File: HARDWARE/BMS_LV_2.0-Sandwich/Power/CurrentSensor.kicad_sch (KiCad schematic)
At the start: 11 parts, among them U5 ACHS-7123

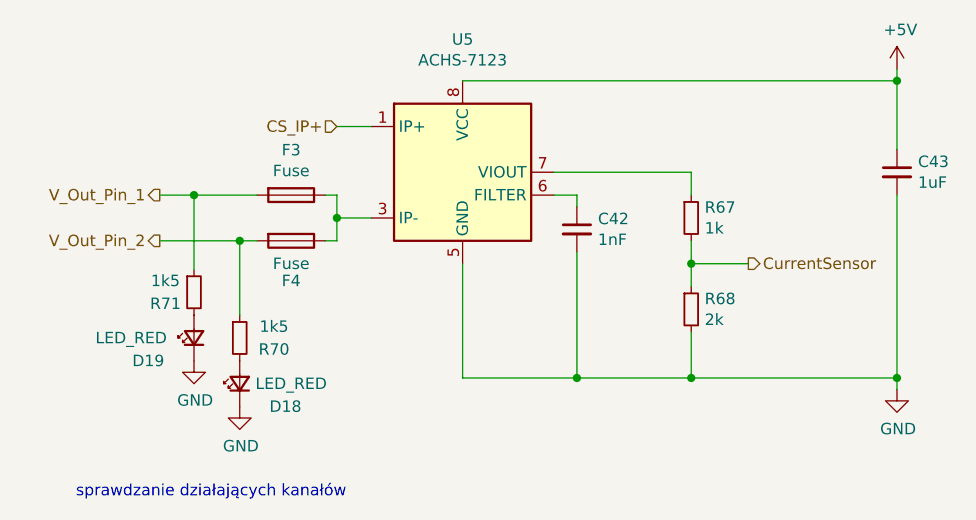
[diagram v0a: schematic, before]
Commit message: Wersja obu plytek gotowa do sprawdzenia
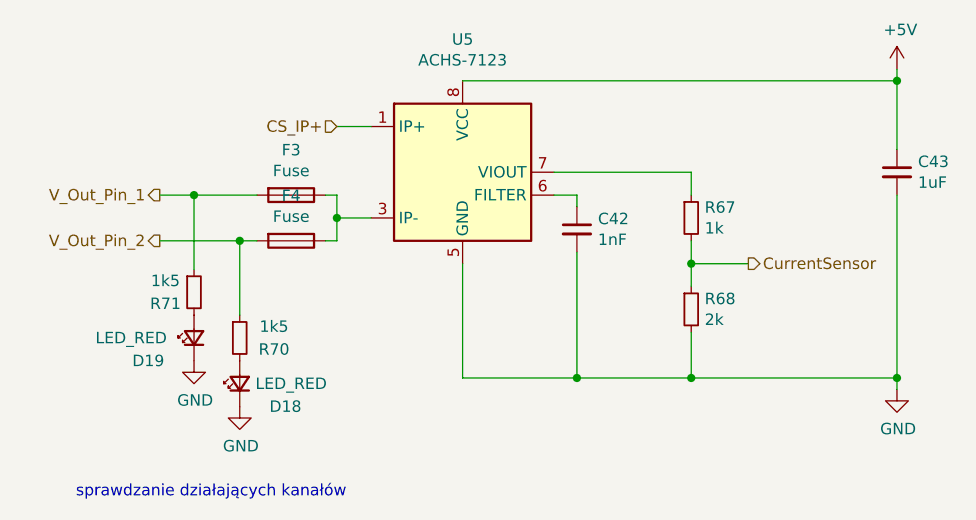
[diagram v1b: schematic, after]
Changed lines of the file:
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@@
+	)
+	(symbol
+		(lib_id "Device:Fuse")
+		(at 118.11 101.6 270)
+		(unit 1)
+		(exclude_from_sim no)
+		(in_bom yes)
+		(on_board yes)
+		(dnp no)
+		(property "Reference" "F4"
+			(at 118.11 96.5962 90)
+			(effects
+				(font
+					(size 1.27 1.27)
+				)
+			)
+		)
+		(property "Value" "Fuse"
+			(at 118.11 98.9076 90)
+			(effects
+				(font
+					(size 1.27 1.27)
+				)
+			)
+		)
+		(property "Footprint" "footprints:FUSC6125X279N"
+			(at 118.11 99.822 90)
+			(effects
+				(font
+					(size 1.27 1.27)
+				)
+				(hide yes)
+			)
+		)
+		(property "Datasheet" "https://www.mouser.pl/ProductDetail/Bel-Fuse/0680L9100-05?qs=XeJtXLiO41RjXNhvn3uPUw%3D%3D"
+			(at 118.11 101.6 0)
+			(effects
+				(font
+					(size 1.27 1.27)
+				)
+				(hide yes)
+			)
+		)
+		(property "Description" "500A interrupt fuse"
+			(at 118.11 101.6 0)
+			(effects
+				(font
+					(size 1.27 1.27)
+				)
+				(hide yes)
+			)
+		)
+		(property "Part Number" "0680L9100-05 "
+			(at 118.11 101.6 0)
+			(effects
+				(font
+					(size 1.27 1.27)
+				)
+				(hide yes)
+			)
+		)
+		(pin "2"
+		)
+		(pin "1"
+		)
+		(instances
+			(project "BMS_LV_2022"
+				(path "/fb6504b5-591d-4b10-ab86-0c46f59e8b7d/00000000-0000-0000-0000-000062c2dd72"
+					(reference "F4")
+					(unit 1)
+				)
+			)
+		)
 	)
 	(symbol
@@
 					(unit 1)
 				)
-			)
-		)
-	)
-	(symbol
-		(lib_id "Device:Fuse")
-		(at 118.11 101.6 270)
-		(unit 1)
-		(exclude_from_sim no)
-		(in_bom yes)
-		(on_board yes)
-		(dnp no)
-		(property "Reference" "F4"
-			(at 118.11 106.045 90)
-			(effects
-				(font
-					(size 1.27 1.27)
-				)
-			)
-		)
-		(property "Value" "Fuse"
-			(at 118.11 104.14 90)
-			(effects
-				(font
-					(size 1.27 1.27)
-				)
-			)
-		)
-		(property "Footprint" "footprints:FUSC6125X279N"
-			(at 118.11 99.822 90)
-			(effects
-				(font
-					(size 1.27 1.27)
-				)
-				(hide yes)
-			)
-		)
-		(property "Datasheet" "https://www.mouser.pl/ProductDetail/Bel-Fuse/0680L9100-05?qs=XeJtXLiO41RjXNhvn3uPUw%3D%3D"
-			(at 118.11 101.6 0)
-			(effects
-				(font
-					(size 1.27 1.27)
-				)
-				(hide yes)
-			)
-		)
-		(property "Description" "500A interrupt fuse"
-			(at 118.11 101.6 0)
-			(effects
-				(font
-					(size 1.27 1.27)
-				)
-				(hide yes)
-			)
-		)
-		(property "Part Number" "0680L9100-05 "
-			(at 118.11 101.6 0)
-			(effects
-				(font
-					(size 1.27 1.27)
-				)
-				(hide yes)
-			)
-		)
-		(pin "2"
-		)
-		(pin "1"
-		)
-		(instances
-			(project "BMS_LV_2022"
-				(path "/fb6504b5-591d-4b10-ab86-0c46f59e8b7d/00000000-0000-0000-0000-000062c2dd72"
-					(reference "F4")
-					(unit 1)
-				)
